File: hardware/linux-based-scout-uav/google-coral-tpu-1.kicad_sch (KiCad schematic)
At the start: 1 part, among them U10 G313-06329-00

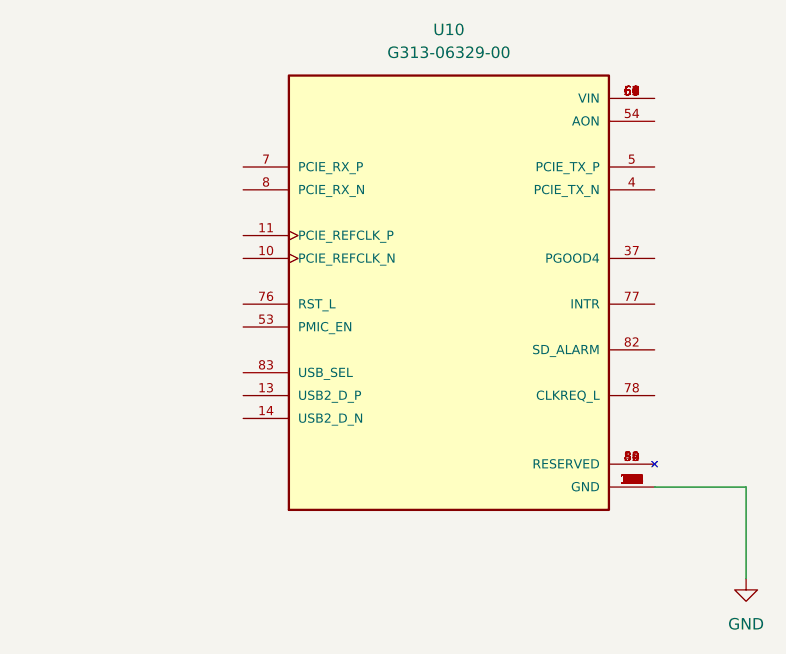
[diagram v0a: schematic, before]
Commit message: Schematic and board update
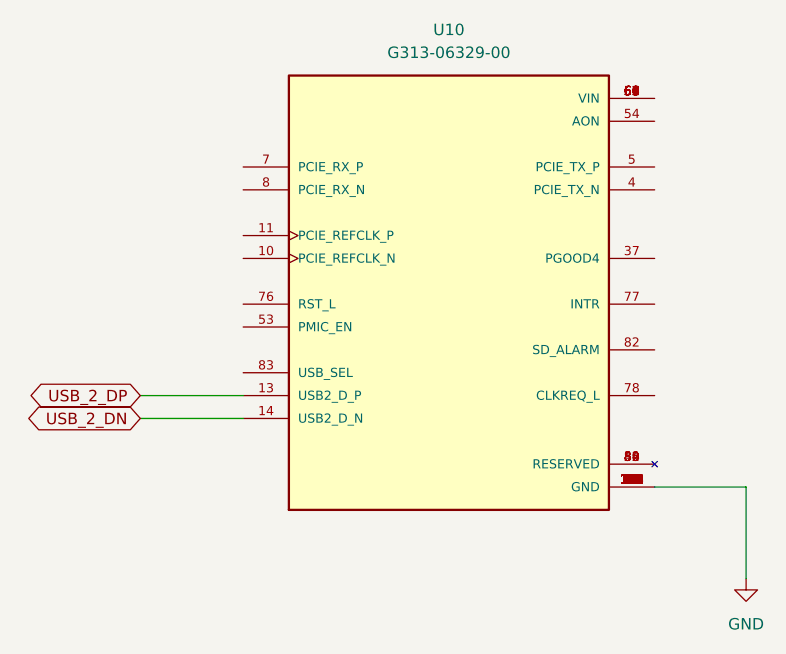
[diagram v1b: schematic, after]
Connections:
- net USB_2_DP: now reaches U10.13 (USB2_D_P)
- net USB_2_DN: now reaches U10.14 (USB2_D_N)
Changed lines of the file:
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@@
+	(wire
+		(pts
+			(xy 168.91 142.24) (xy 180.34 142.24)
+		)
+		(stroke
+			(width 0)
+			(type default)
+		)
+	)
 	(wire
 		(pts
@@
 		)
 	)
+	(wire
+		(pts
+			(xy 168.91 139.7) (xy 180.34 139.7)
+		)
+		(stroke
+			(width 0)
+			(type default)
+		)
+	)
+	(global_label "USB_2_DN"
+		(shape bidirectional)
+		(at 168.91 142.24 180)
+		(fields_autoplaced yes)
+		(effects
+			(font
+				(size 1.27 1.27)
+			)
+			(justify right)
+		)
+		(property "Intersheetrefs" "${INTERSHEET_REFS}"
+			(at 155.2583 142.24 0)
+			(effects
+				(font
+					(size 1.27 1.27)
+				)
+				(justify right)
+				(hide yes)
+			)
+		)
+	)
+	(global_label "USB_2_DP"
+		(shape bidirectional)
+		(at 168.91 139.7 180)
+		(fields_autoplaced yes)
+		(effects
+			(font
+				(size 1.27 1.27)
+			)
+			(justify right)
+		)
+		(property "Intersheetrefs" "${INTERSHEET_REFS}"
+			(at 155.3188 139.7 0)
+			(effects
+				(font
+					(size 1.27 1.27)
+				)
+				(justify right)
+				(hide yes)
+			)
+		)
+	)
